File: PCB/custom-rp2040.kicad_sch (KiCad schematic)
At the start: 34 parts, among them J1 USB_C_Receptacle_USB2.0, J2 SWD, SW1 SW_Push, U1 W25Q128JVS, U2 USBLC6-2SC6, U3 RP2040, U4 AMS1117-3.3, Y1 12MHz

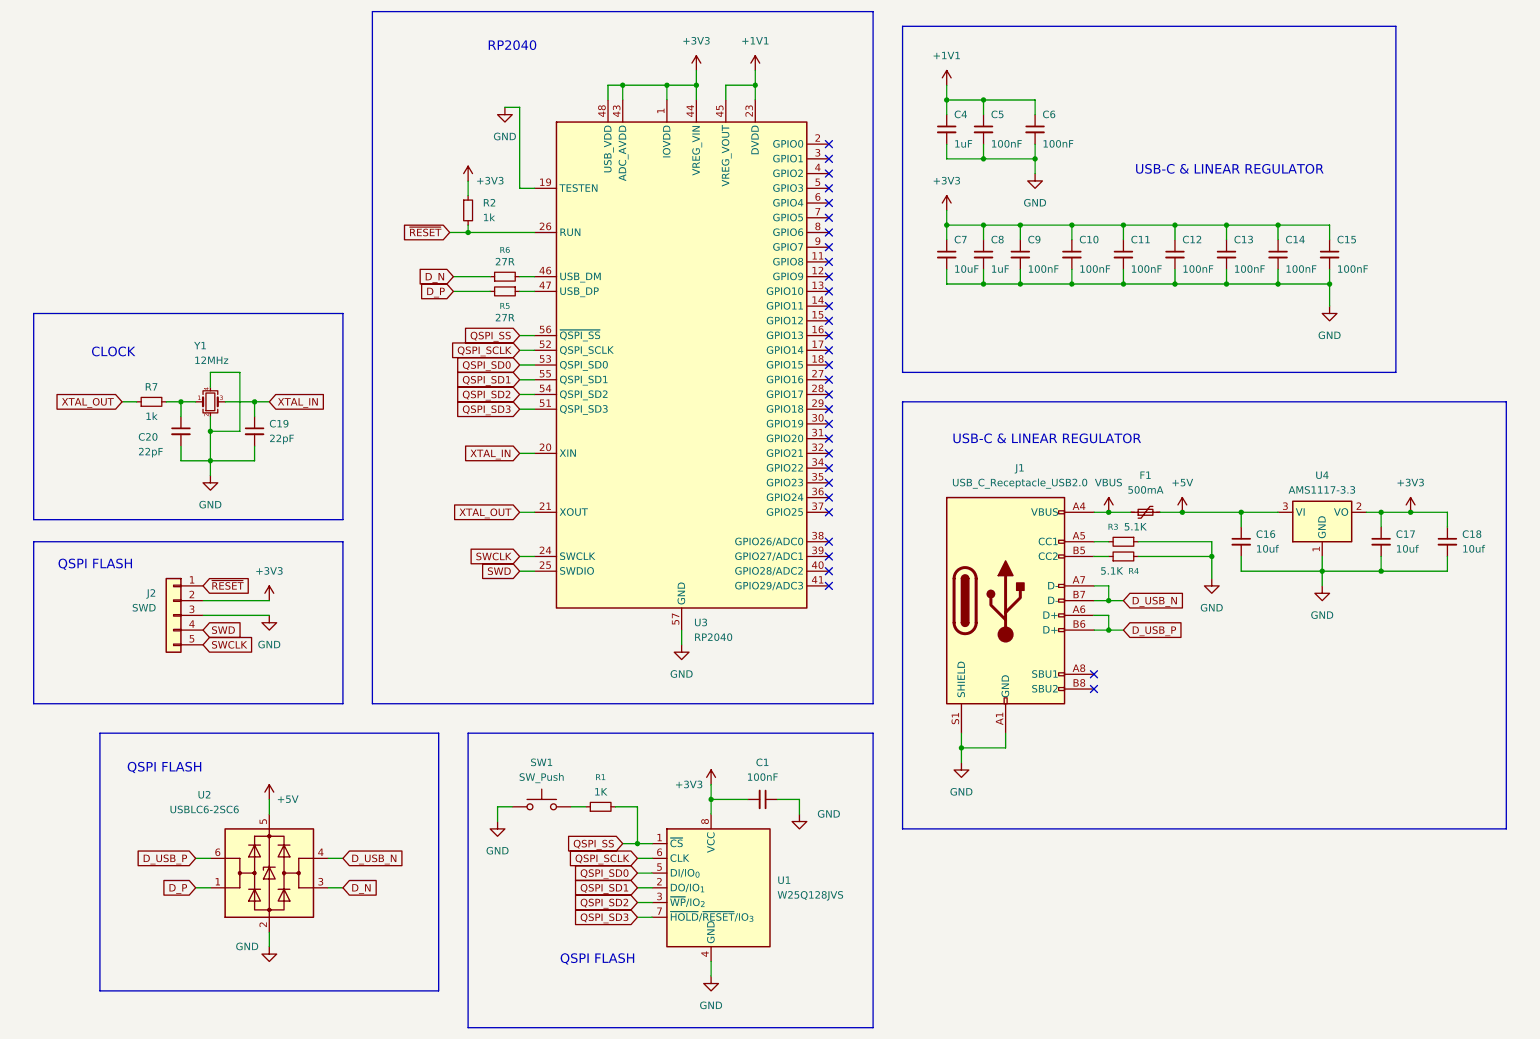
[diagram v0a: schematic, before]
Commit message: Layout board
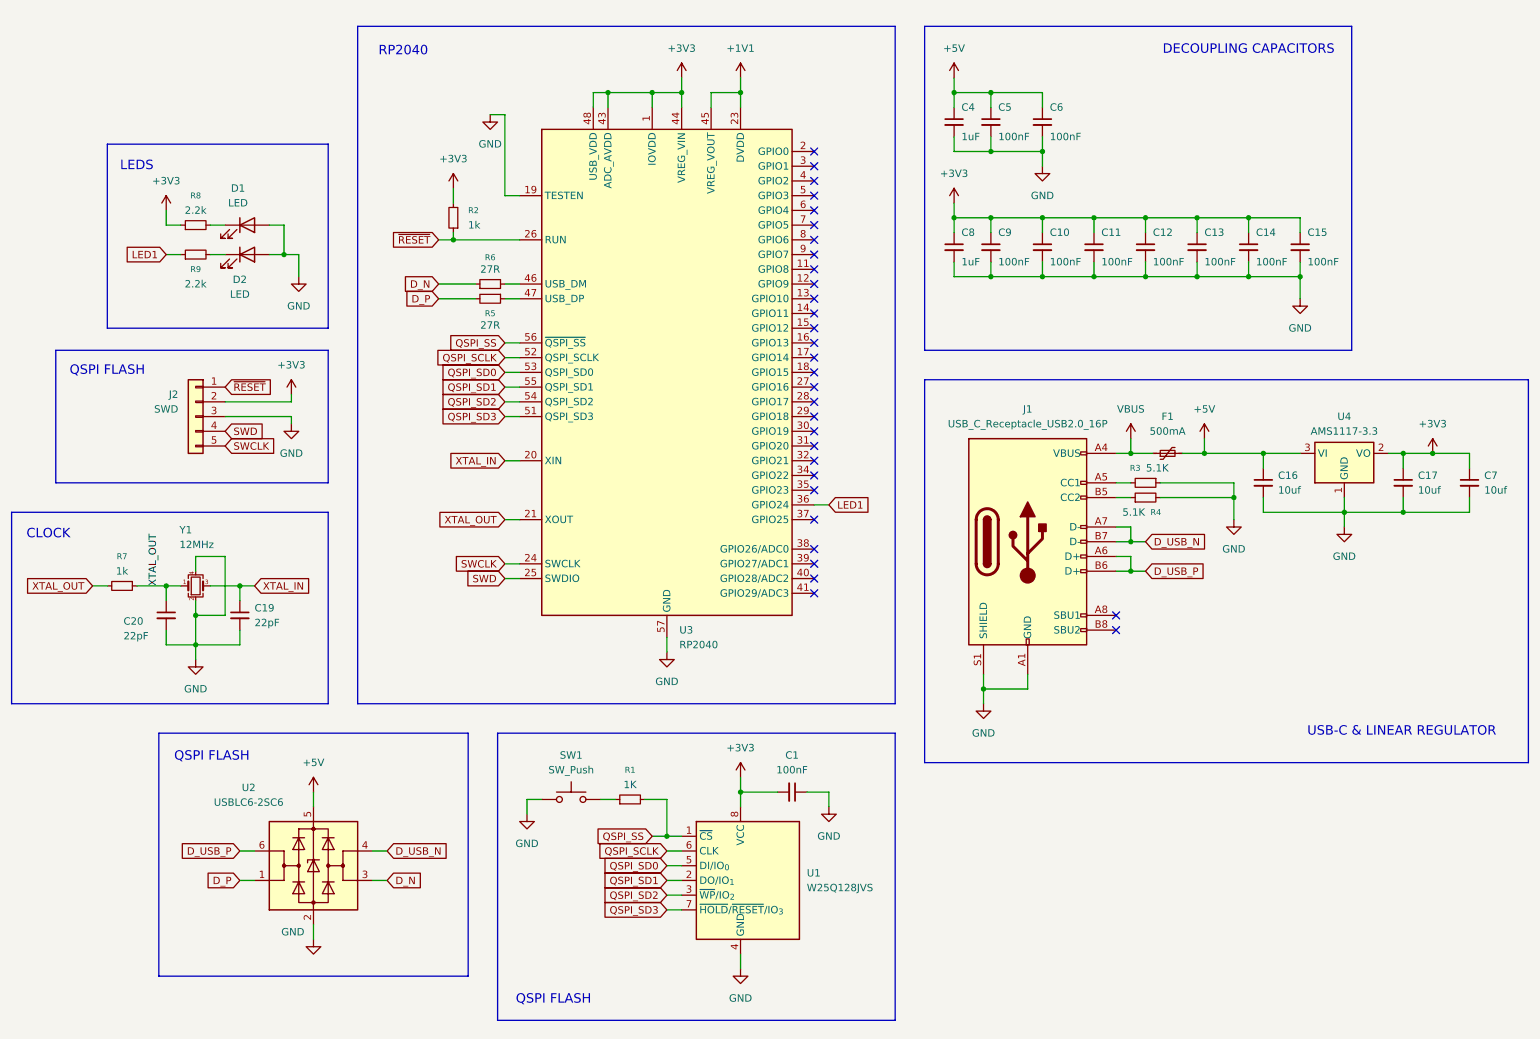
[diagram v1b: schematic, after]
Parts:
- removed C7: 10uF, Capacitor_SMD:C_0402_1005Metric, symbol Device:C_Small
- removed J1: USB_C_Receptacle_USB2.0, Connector_USB:USB_C_Receptacle_HRO_TYPE-C-31-M-12, symbol Connector:USB_C_Receptacle_USB2.0
- added D1, D2: LED, LED_SMD:LED_0402_1005Metric, symbol Device:LED
- added J1: USB_C_Receptacle_USB2.0_16P, Connector_USB:USB_C_Receptacle_HCTL_HC-TYPE-C-16P-01A, symbol Connector:USB_C_Receptacle_USB2.0_16P
- added R8, R9: 2.2k, Resistor_SMD:R_0402_1005Metric, symbol Device:R_Small
- C1, C16, C17, C19, C20: footprint (none) -> Capacitor_SMD:C_0402_1005Metric
- C7: renamed from C18; footprint (none) -> Capacitor_SMD:C_0402_1005Metric
- F1: LCSC C70076 -> (none)
- R1, R3, R4, R5, R6: footprint (none) -> Resistor_SMD:R_0402_1005Metric
- R2, R7: LCSC C11702 -> (none)
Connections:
- net +1V1: no longer C4.1, C5.1, C6.1
- net +3V3: now also R2.2, R8.1; no longer R2.1
- net +5V: now also C4.1, C5.1, C6.1
- net D_USB_N: now also J1.A7 (D-), J1.B7 (D-)
- net D_USB_P: now also J1.A6 (D+), J1.B6 (D+)
- net GND: now also D1.2 (A), D2.2 (A), J1.A1 (GND), J1.A12 (GND), J1.B1 (GND), J1.B12 (GND), J1.S1 (SHIELD)
- net VBUS: now also J1.A4 (VBUS), J1.A9 (VBUS), J1.B4 (VBUS), J1.B9 (VBUS)
- net XTAL_OUT: now also C20.1, R7.2, Y1.1
- net ~{RESET}: now also R2.1; no longer R2.2
- net at R3.2: now also J1.A5 (CC1)
- net LED1: now reaches U3.36 (GPIO24)
- net LED1: now also R9.1
- net at R4.1: now also J1.B5 (CC2)
- new net: D2.1 (K), R9.2
- new net: D1.1 (K), R8.2
- no-connect marks 32 -> 31
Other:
- note added: "DECOUPLING CAPACITORS"
- note added: "LEDS"
- company: (none) -> ImSeanConroy
- title: (none) -> Custom RP2040
- moved on the sheet: C1, C10, C11, C12, C13, C14, C15, C16, C17, C19, C20, C4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
